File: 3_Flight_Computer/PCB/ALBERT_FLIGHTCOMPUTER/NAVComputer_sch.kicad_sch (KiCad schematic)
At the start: 28 parts, among them J11 USB_C_Receptacle_USB2.0_14P, J15 Conn_01x08, J16 Conn_01x05, SW2 SW_SPDT, Y2 16MHz

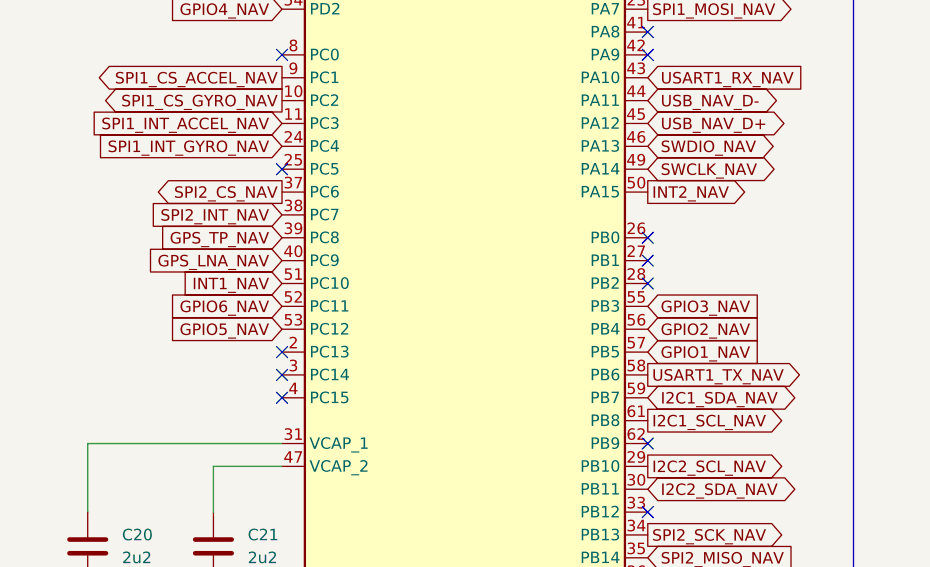
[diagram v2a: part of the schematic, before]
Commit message: update pcb
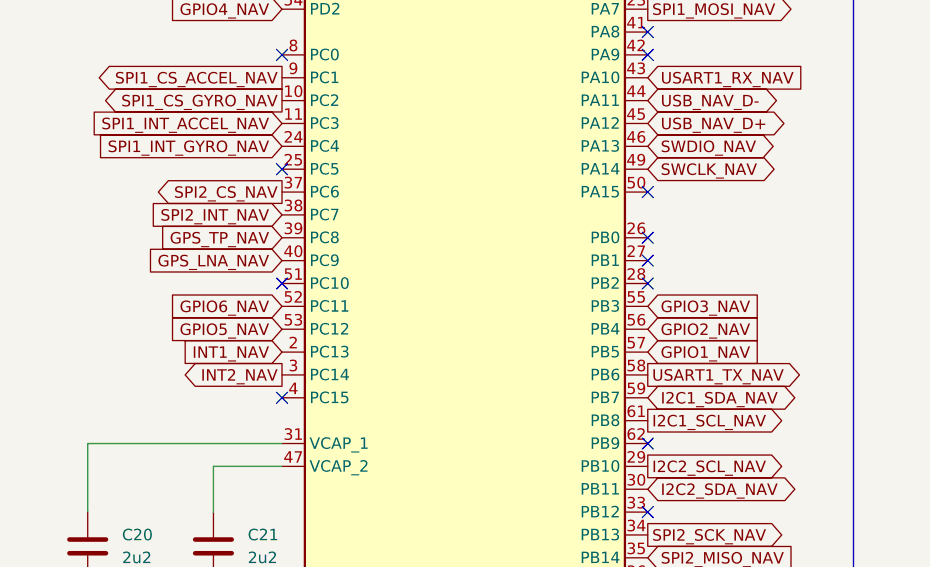
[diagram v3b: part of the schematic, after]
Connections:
- net INT1_NAV: now also NAV1.2 (PC13); no longer NAV1.51 (PC10)
- net INT2_NAV: now also NAV1.3 (PC14); no longer NAV1.50 (PA15)
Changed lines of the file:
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@@
+	)
+	(no_connect
+		(at 97.79 86.36)
 	)
 	(no_connect
@@
 	)
 	(no_connect
+		(at 57.15 96.52)
+	)
+	(no_connect
 		(at 57.15 71.12)
-	)
-	(no_connect
-		(at 57.15 104.14)
 	)
 	(no_connect
@@
 	(no_connect
 		(at 97.79 50.8)
-	)
-	(no_connect
-		(at 57.15 106.68)
 	)
 	(wire
@@
 		)
 	)
-	(global_label "INT1_NAV"
-		(shape input)
-		(at 57.15 96.52 180)
-		(fields_autoplaced yes)
-		(effects
-			(font
-				(size 1.27 1.27)
-			)
-			(justify right)
-		)
-		(property "Intersheetrefs" "${INTERSHEET_REFS}"
-			(at 45.5771 96.52 0)
+	(global_label "INT2_NAV"
+		(shape output)
+		(at 57.15 106.68 180)
+		(fields_autoplaced yes)
+		(effects
+			(font
+				(size 1.27 1.27)
+			)
+			(justify right)
+		)
+		(property "Intersheetrefs" "${INTERSHEET_REFS}"
+			(at 45.5771 106.68 0)
 			(effects
 				(font
@@
 		)
 	)
+	(global_label "INT1_NAV"
+		(shape input)
+		(at 57.15 104.14 180)
+		(fields_autoplaced yes)
+		(effects
+			(font
+				(size 1.27 1.27)
+			)
+			(justify right)
+		)
+		(property "Intersheetrefs" "${INTERSHEET_REFS}"
+			(at 45.5771 104.14 0)
+			(effects
+				(font
+					(size 1.27 1.27)
+				)
+				(justify right)
+				(hide yes)
+			)
+		)
+	)
 	(global_label "GPIO3_NAV"
 		(shape input)
@@
 				(hide yes)
 			)
-		)
-	)
-	(global_label "INT2_NAV"
-		(shape output)
-		(at 97.79 86.36 0)
-		(fields_autoplaced yes)
-		(effects
-			(font
-				(size 1.27 1.27)
-			)
-			(justify left)
-		)
-		(property "Intersheetrefs" "${INTERSHEET_REFS}"
-			(at 109.3629 86.36 0)
-			(effects
-				(font
-					(size 1.27 1.27)
-				)
-				(justify left)
-				(hide yes)
-			)
